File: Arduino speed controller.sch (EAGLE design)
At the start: 13 parts, among them J1 AUDIO-JACK2KIT, J2 AUDIO-JACK2KIT

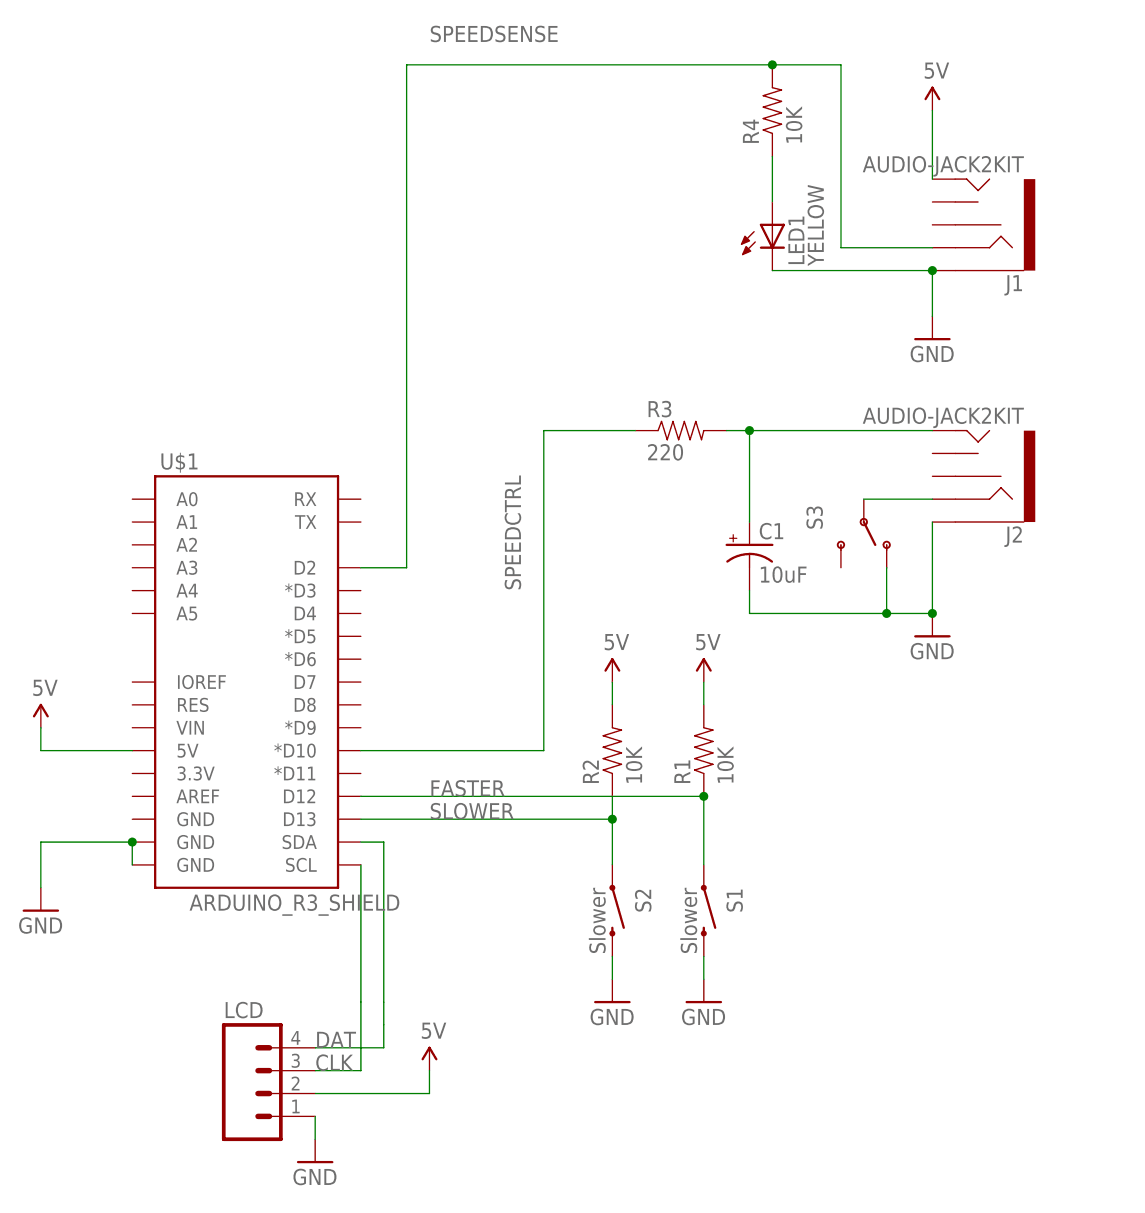
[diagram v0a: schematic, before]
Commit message: Added DAC
Added DAC
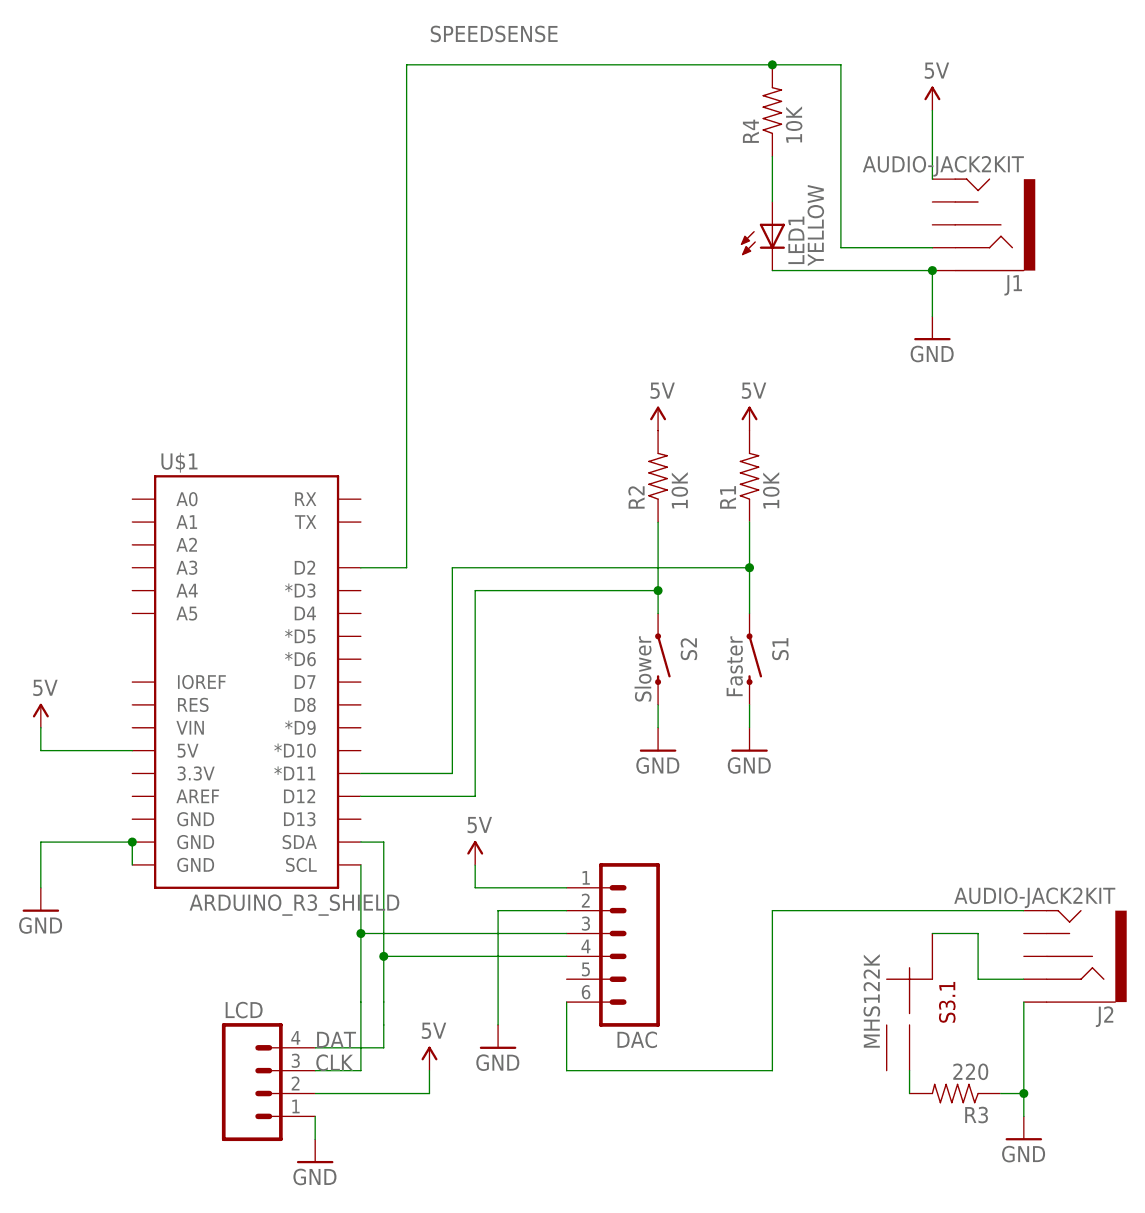
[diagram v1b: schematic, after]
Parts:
- removed C1: 10uF, SparkFun-Passives:CAP_POLPTH2
- added DAC: (no value), SparkFun-Connectors:M06SIP
- S1: value Slower -> Faster
- S3: value (none) -> MHS122K; device SparkFun-Electromechanical:SWITCH-SPDTKIT -> switches:MHS122K
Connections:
- removed net N$4: C1.+, J2.TIP, R3.2
- removed net SPEEDCTRL: R3.1, U$1.*D10
- new net N$1: J2.RING, S3.1.CM
- new net N$3: DAC.6, J2.TIP
- net 5V: now also DAC.1
- net CLK: now also DAC.3
- net DAT: now also DAC.4
- net FASTER: now also U$1.*D11; no longer U$1.D12
- net GND: now also DAC.2, R3.1; no longer C1.-, S3.O
- net N$2: now also R3.2, S3.1.1; no longer J2.RING, S3.P
- net SLOWER: now also U$1.D12; no longer U$1.D13
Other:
- moved on the sheet: J2, R1, R2, R3, S1, S2
